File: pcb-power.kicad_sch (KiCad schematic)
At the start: 19 parts, among them J1 Conn_01x07_Socket, J2 Conn_01x02_Socket, J3 Conn_01x02_Socket, Q1 PMOS, Q2 NMOS, Q3 PMOS, Q4 PMOS, Q5 NMOS, Q6 NMOS, U1 LM1117MP-3.3, U2 LM1117MP-3.3

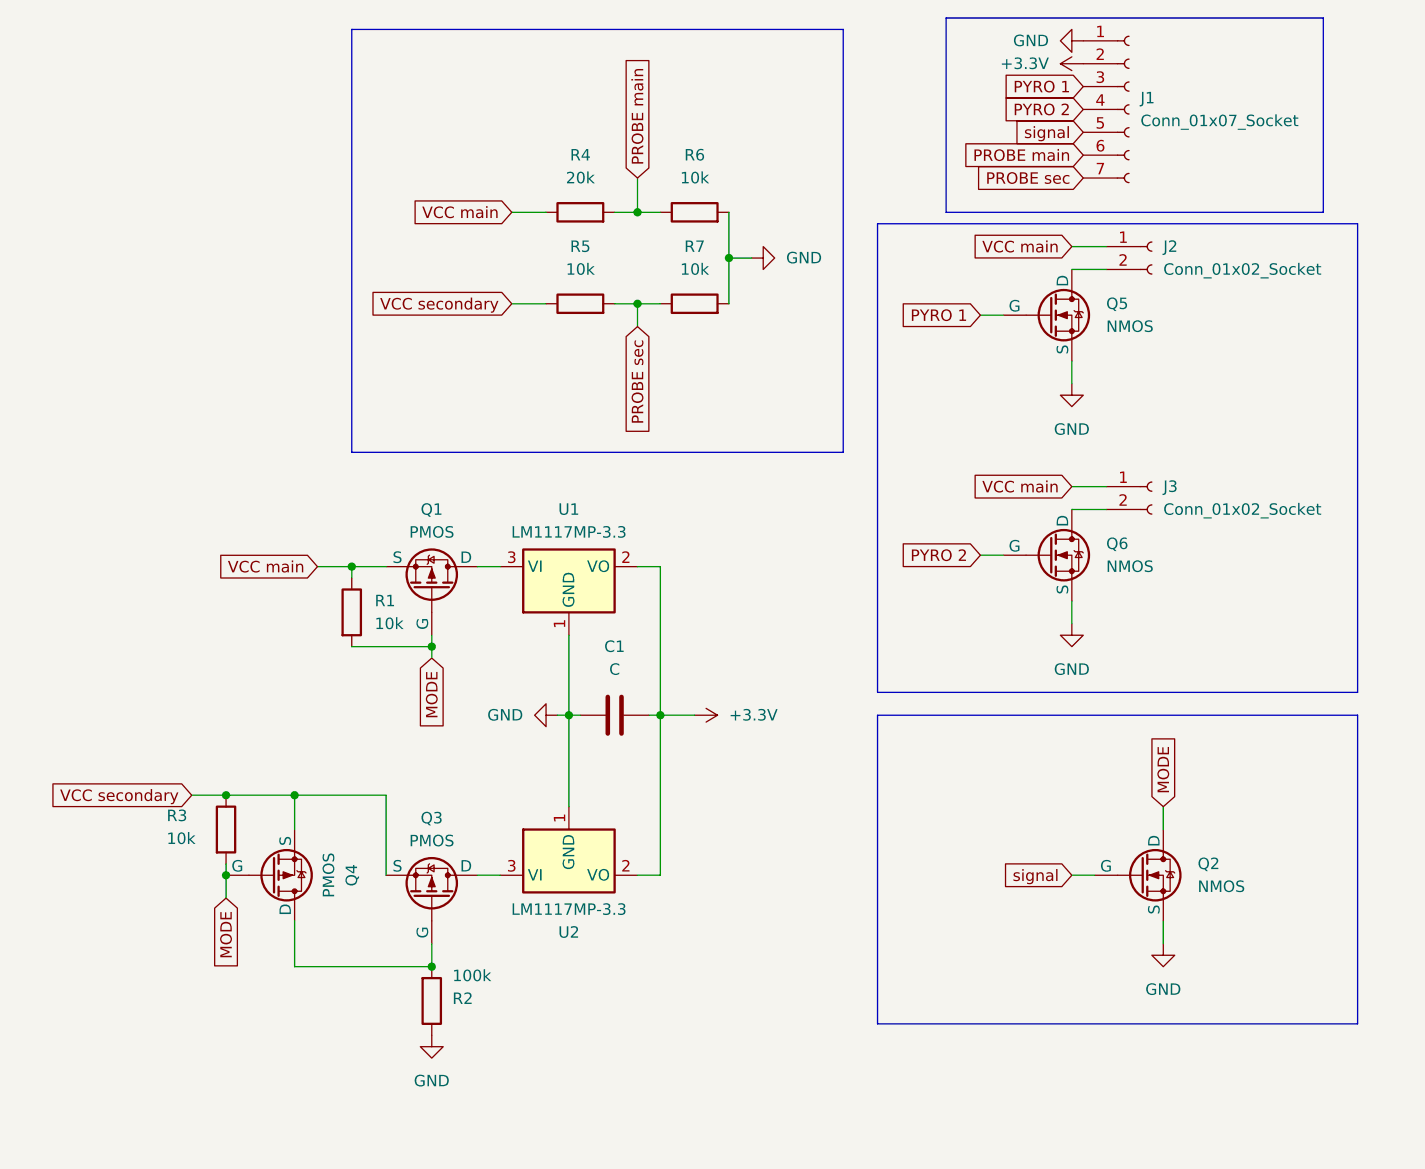
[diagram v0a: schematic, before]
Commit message: pcb design done
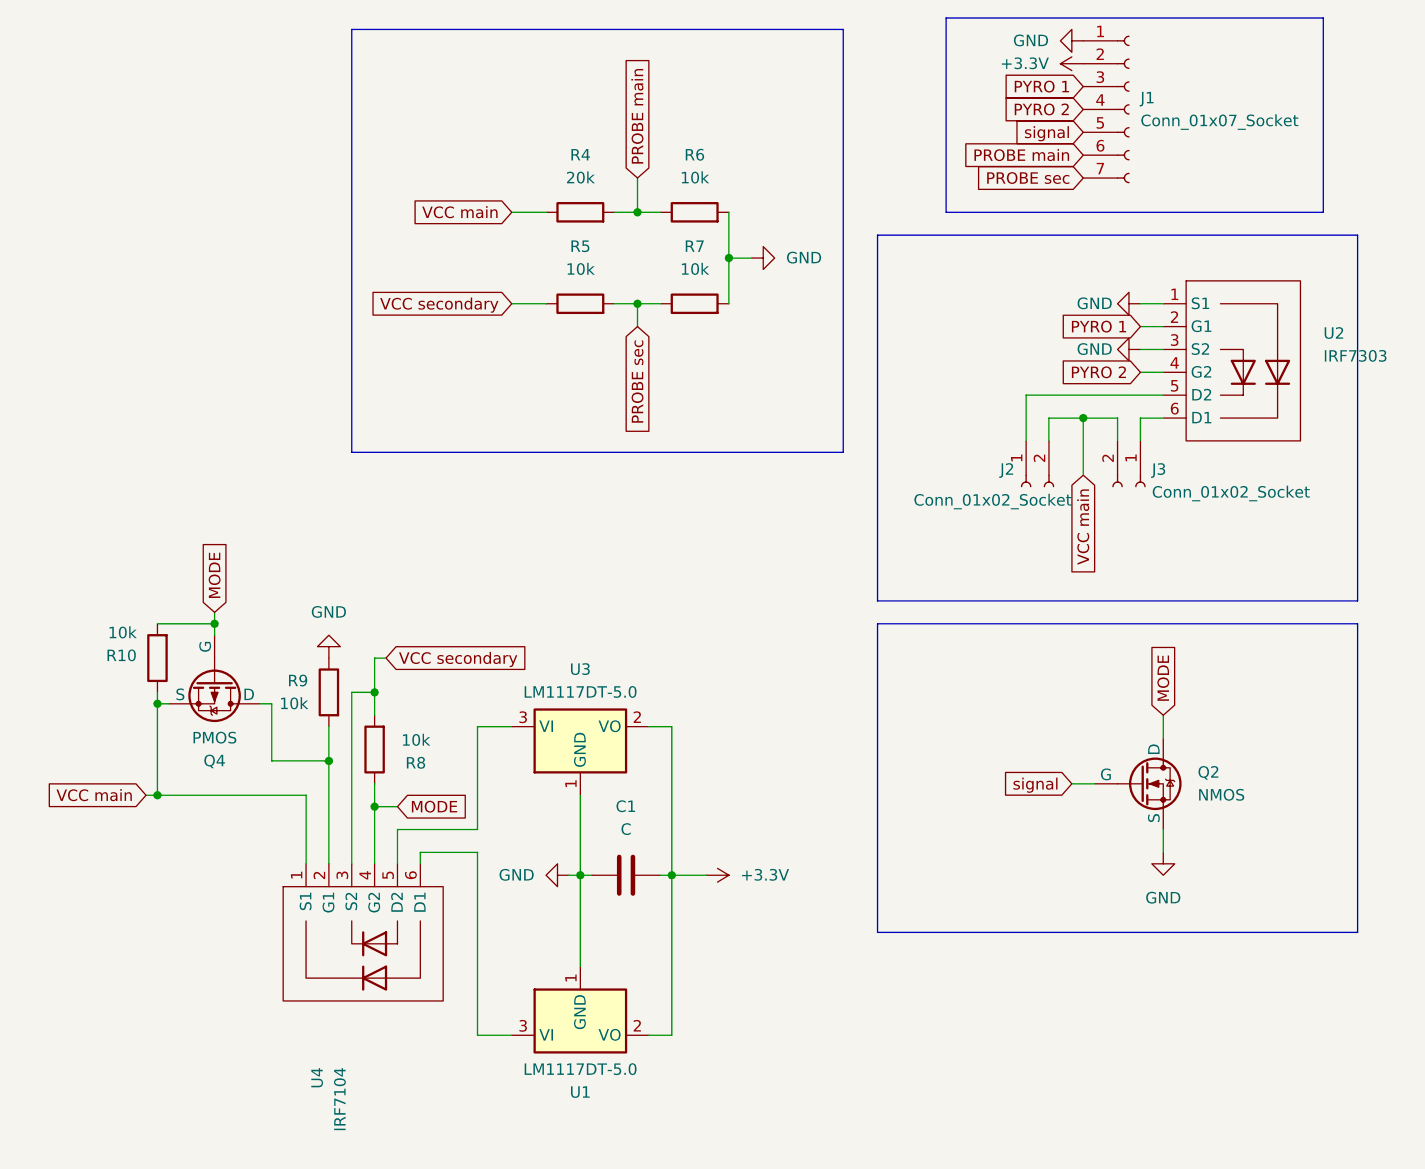
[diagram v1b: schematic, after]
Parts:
- removed Q1, Q3: PMOS, symbol Simulation_SPICE:PMOS
- removed Q5, Q6: NMOS, symbol Simulation_SPICE:NMOS
- removed R1, R3: 10k, symbol Device:R
- removed R2: 100k, symbol Device:R
- removed U1, U2: LM1117MP-3.3, Package_TO_SOT_SMD:SOT-223-3_TabPin2, symbol Regulator_Linear:LM1117MP-3.3
- added R10, R8, R9: 10k, Resistor_THT:R_Axial_DIN0207_L6.3mm_D2.5mm_P10.16mm_Horizontal, symbol Device:R
- added U1, U3: LM1117DT-5.0, Package_TO_SOT_SMD:TO-252-3_TabPin2, symbol Regulator_Linear:LM1117DT-5.0
- added U2: IRF7303, Package_TO_SOT_SMD:IRF7303, symbol Transistor_FET:IRF7303
- added U4: IRF7104, Package_TO_SOT_SMD:IRF7104, symbol Transistor_FET:IRF7104
- C1: footprint (none) -> Capacitor_THT:CP_Radial_D5.0mm_P2.00mm
- J1: footprint (none) -> Connector_PinSocket_2.54mm:PinSocket_1x07_P2.54mm_Vertical
- J2, J3: footprint (none) -> ark:TerminalBlock_bornier-2_P5.08mm
- Q2: footprint (none) -> Package_TO_SOT_SMD:SOT-23
- Q4: footprint (none) -> Package_TO_SOT_SMD:TO-252-2
- R4, R5, R6, R7: footprint (none) -> Resistor_THT:R_Axial_DIN0207_L6.3mm_D2.5mm_P10.16mm_Horizontal
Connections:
- net +3.3V: now also U1.2 (VO), U3.2 (VO)
- net GND: now also R9.1, U1.1 (GND), U2.1 (S1), U2.3 (S2), U3.1 (GND)
- net MODE: now also R10.2, R8.1, U4.4 (G2)
- net PYRO 1: now also U2.2 (G1)
- net PYRO 2: now also U2.4 (G2)
- net VCC main: now also J2.2 (Pin_2), J3.2 (Pin_2), Q4.3 (S), R10.1, U4.1 (S1); no longer J2.1 (Pin_1), J3.1 (Pin_1)
- net VCC secondary: now also R8.2, U4.3 (S2); no longer Q4.3 (S)
- net at Q4.1 (D): now also R9.2, U4.2 (G1)
- new net: J2.1 (Pin_1), U2.5 (D2)
- new net: J3.1 (Pin_1), U2.6 (D1)
- new net: U3.3 (VI), U4.5 (D2)
- new net: U1.3 (VI), U4.6 (D1)
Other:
- moved on the sheet: C1, J2, J3, Q2
